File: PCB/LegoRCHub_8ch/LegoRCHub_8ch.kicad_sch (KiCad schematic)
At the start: 31 parts, among them J1 Conn_01x02, J10 Conn_01x02, J11 Conn_01x03, J2 Conn_01x02, J3 Conn_01x02, J4 Conn_01x02, J5 Conn_01x03, J6 Conn_01x03, J7 Conn_01x03, J8 Conn_01x03, J9 Conn_01x02, U1 DRV8872DDA, U2 DRV8872DDA, U3 DRV8872DDA, U4 DRV8872DDA, U6 AMS1117-5.0, U7 ATtiny3226-X

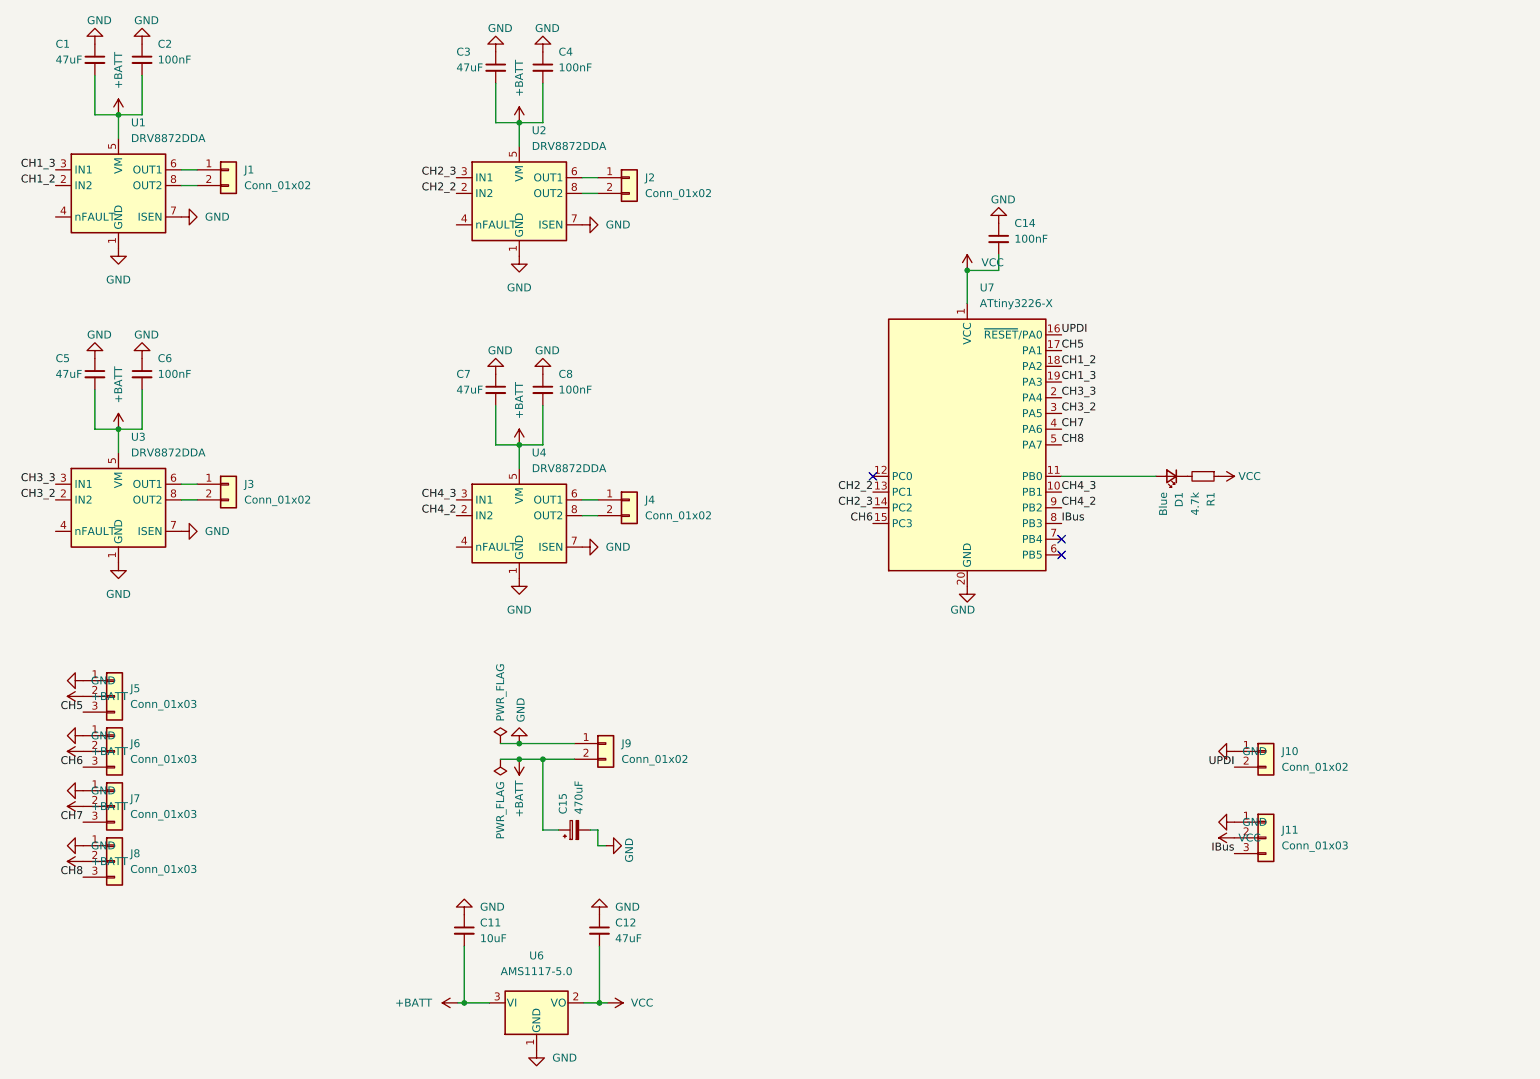
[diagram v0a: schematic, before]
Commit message: ...
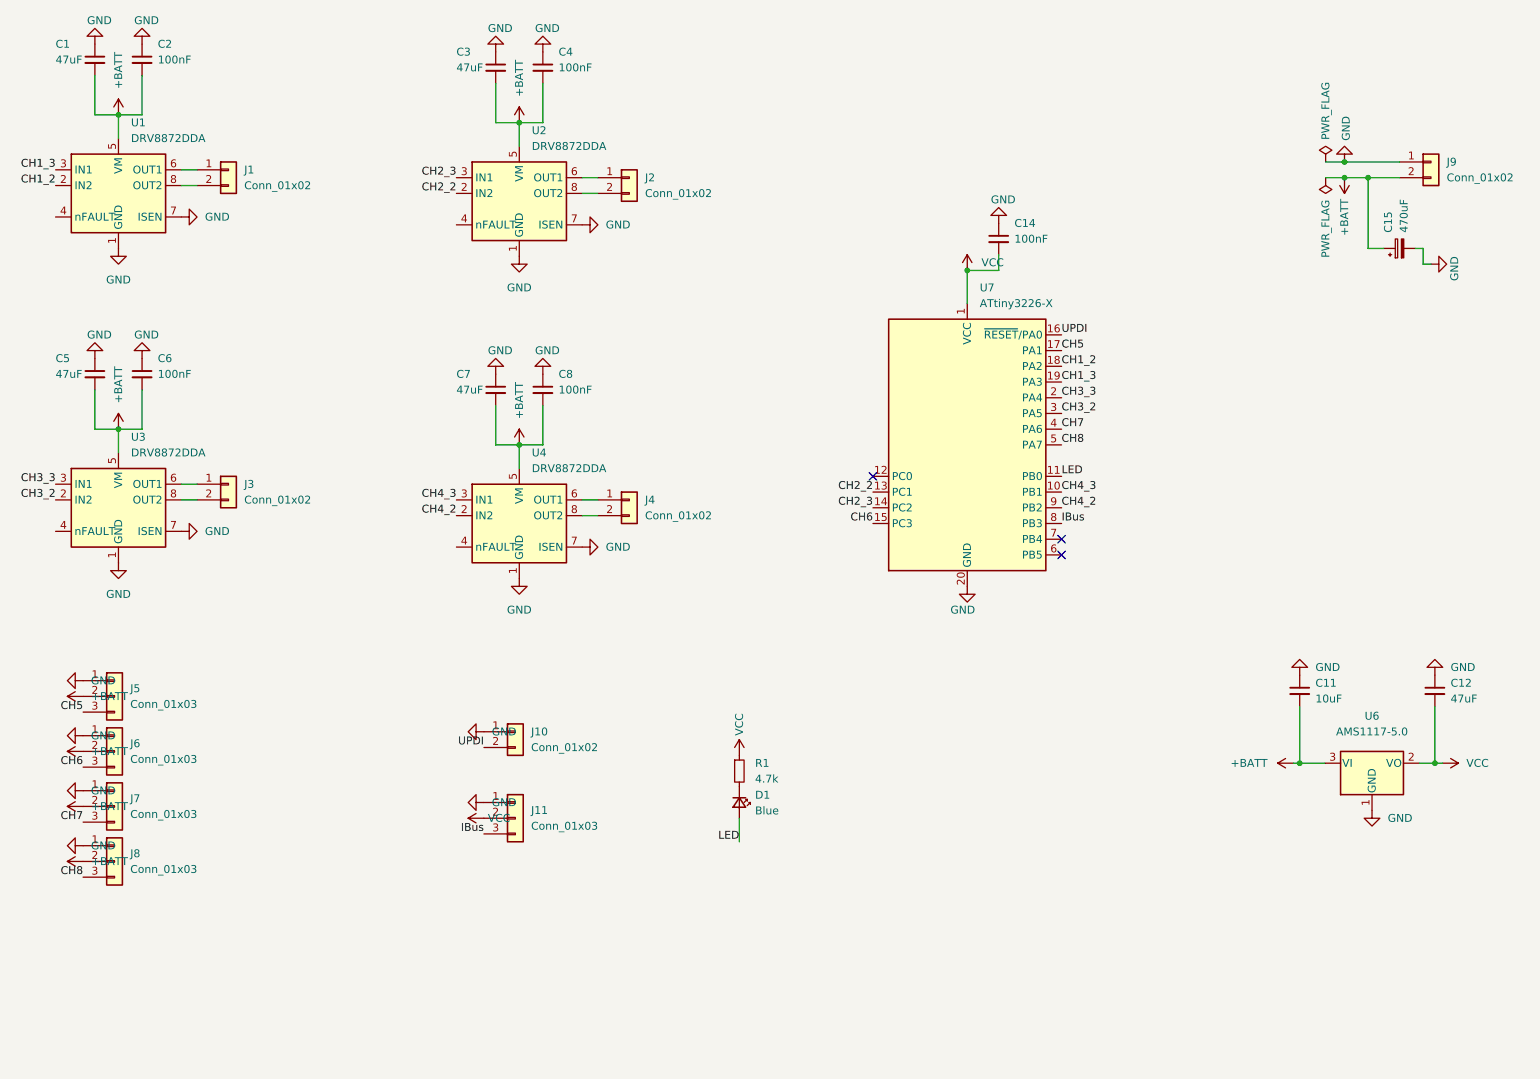
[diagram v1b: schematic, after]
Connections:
- net LED: now reaches D1.2 (A), U7.11 (PB0)
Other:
- moved on the sheet: C11, C12, C15, D1, J10, J11, J9, R1, U6
